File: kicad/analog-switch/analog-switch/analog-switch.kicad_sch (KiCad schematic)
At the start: 12 parts, among them J1 Conn_01x04, J2 Conn_01x16_MountingPin, J3 Conn_02x01_Row_Letter_First, J4 Conn_01x04, J5 Conn_01x16_MountingPin, Q1 Q_PNP_EBC, U1 CD74HC4067M, U2 74HC595, U3 CD74HC4067M

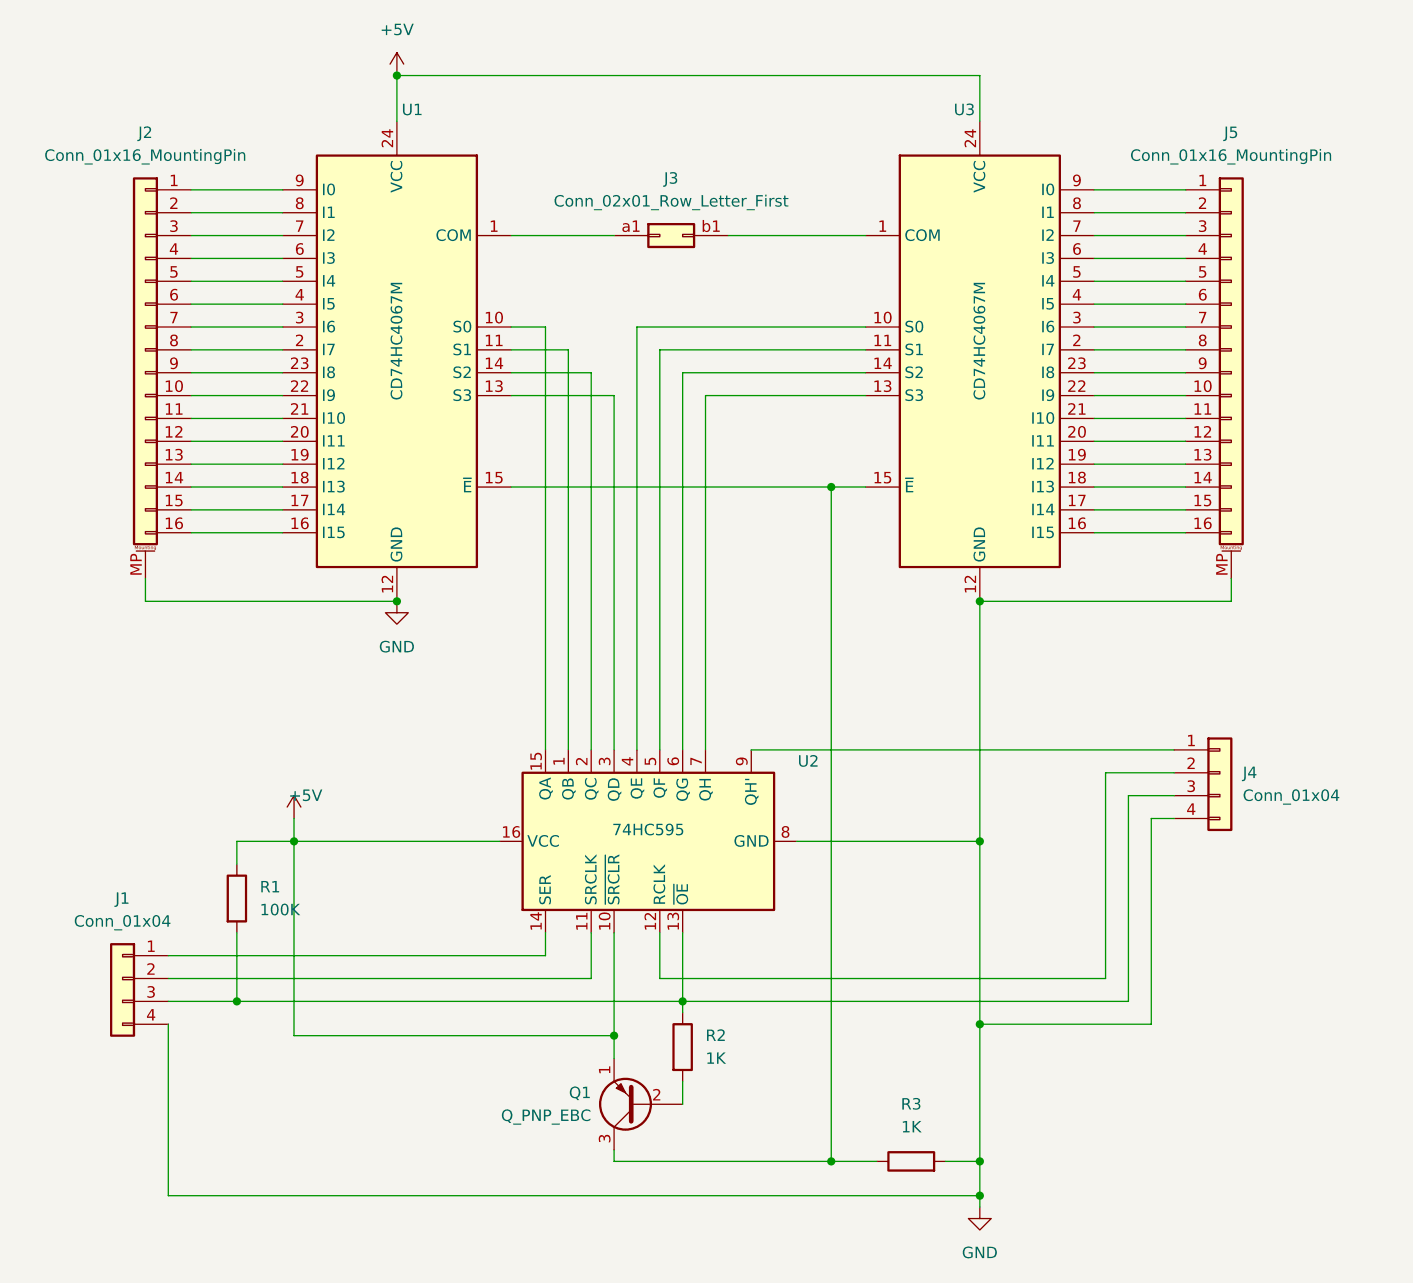
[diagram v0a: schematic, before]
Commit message: proj settings
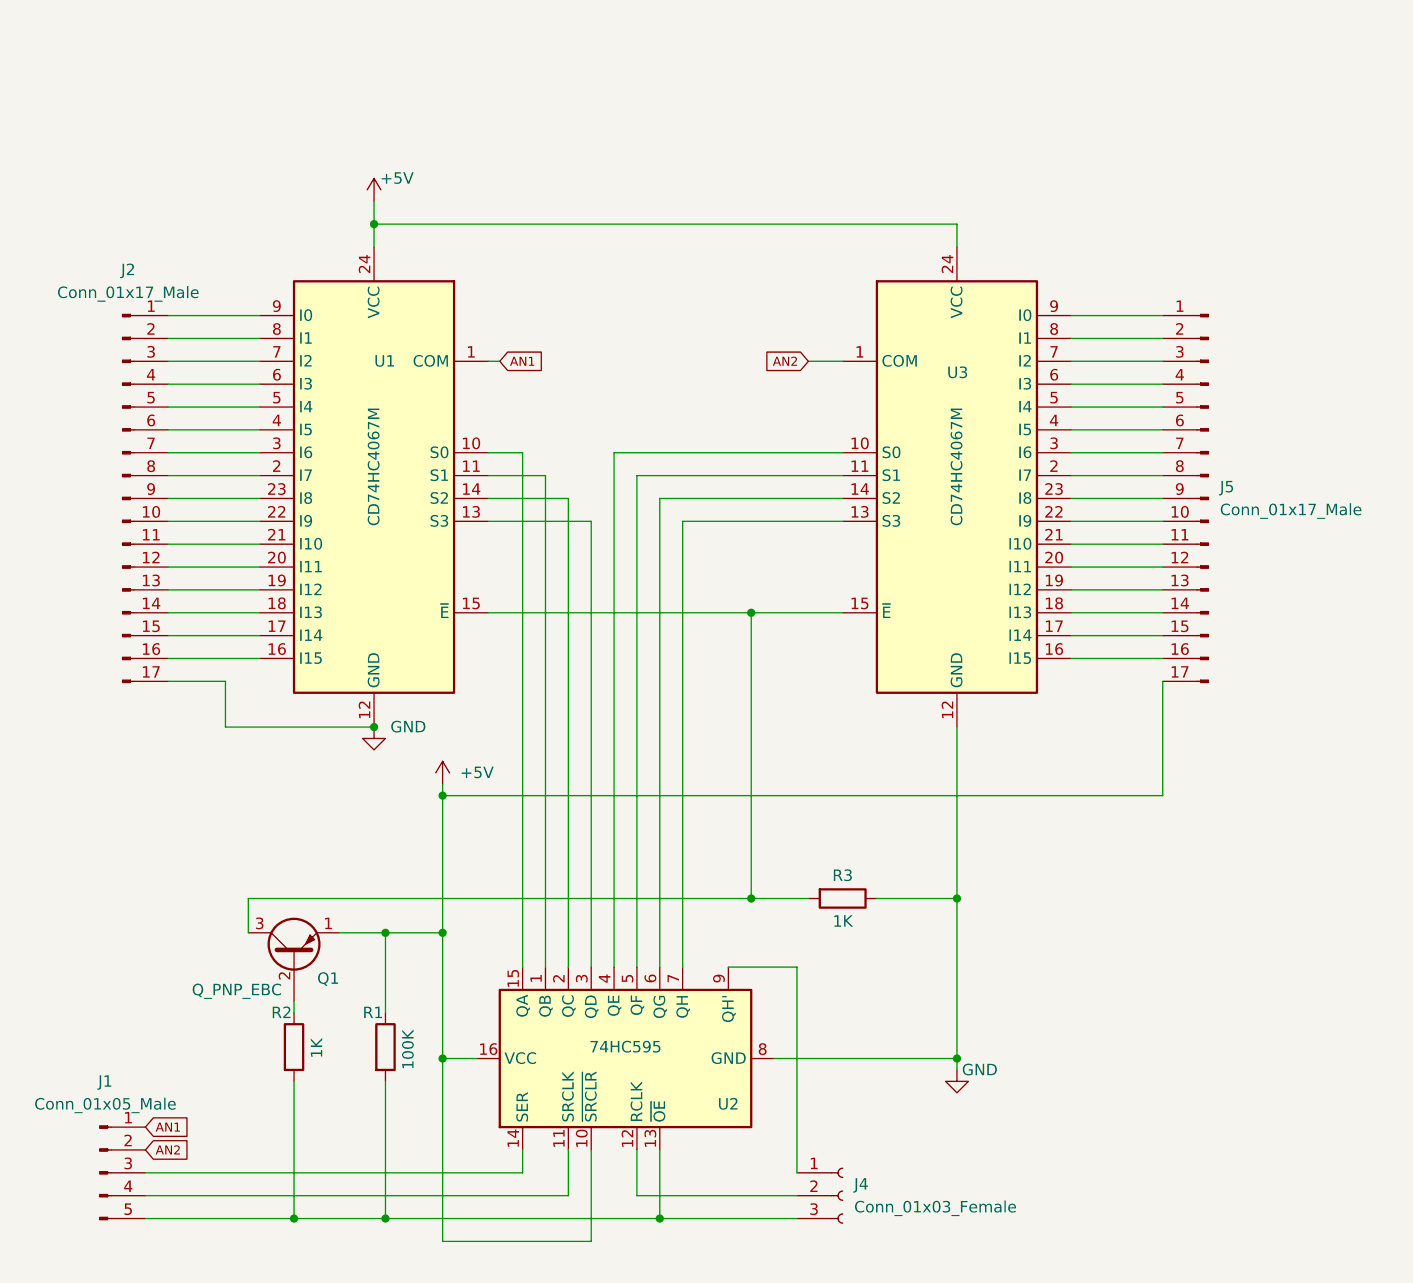
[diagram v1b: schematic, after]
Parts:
- removed J1, J4: Conn_01x04, Connector_PinHeader_2.54mm:PinHeader_1x04_P2.54mm_Vertical, symbol Connector_Generic:Conn_01x04
- removed J2, J5: Conn_01x16_MountingPin, Connector_PinHeader_2.54mm:PinHeader_1x16_P2.54mm_Vertical, symbol Connector_Generic_MountingPin:Conn_01x16_MountingPin
- removed J3: Conn_02x01_Row_Letter_First, symbol Connector_Generic:Conn_02x01_Row_Letter_First
- added J1: Conn_01x05_Male, Connector_PinHeader_2.00mm:PinHeader_1x05_P2.00mm_Vertical, symbol Connector:Conn_01x05_Male
- added J2, J5: Conn_01x17_Male, Connector_PinHeader_2.54mm:PinHeader_1x17_P2.54mm_Vertical, symbol Connector:Conn_01x17_Male
- added J4: Conn_01x03_Female, Connector_PinHeader_2.00mm:PinHeader_1x03_P2.00mm_Vertical, symbol Connector:Conn_01x03_Female
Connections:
- net +5V: now also J5.17 (Pin_17)
- net GND: now also R3.1, J2.17 (Pin_17); no longer R3.2
- net at U2.9 (QH'): now also J4.1 (Pin_1)
- net at U2.12 (RCLK): now also J4.2 (Pin_2)
- net at R1.2, U2.13 (~{OE}): now also R2.2, J1.5 (Pin_5), J4.3 (Pin_3); no longer R2.1
- net AN2: now reaches U3.1 (COM)
- net AN2: now also J1.2 (Pin_2)
- net at Q1.3 (C), U1.15 (~{E}), U3.15 (~{E}): now also R3.2; no longer R3.1
- net at U3.16 (I15): now also J5.16 (Pin_16)
- net at U3.17 (I14): now also J5.15 (Pin_15)
- net at U3.18 (I13): now also J5.14 (Pin_14)
- net at U3.19 (I12): now also J5.13 (Pin_13)
- net at U3.2 (I7): now also J5.8 (Pin_8)
- net at U3.20 (I11): now also J5.12 (Pin_12)
- net at U3.21 (I10): now also J5.11 (Pin_11)
- net at U3.22 (I9): now also J5.10 (Pin_10)
- net at U3.23 (I8): now also J5.9 (Pin_9)
- net at U3.3 (I6): now also J5.7 (Pin_7)
- net at U3.4 (I5): now also J5.6 (Pin_6)
- net at U3.5 (I4): now also J5.5 (Pin_5)
- net at U3.6 (I3): now also J5.4 (Pin_4)
- net at U3.7 (I2): now also J5.3 (Pin_3)
- net at U3.8 (I1): now also J5.2 (Pin_2)
- net at U3.9 (I0): now also J5.1 (Pin_1)
- net AN1: now reaches U1.1 (COM)
- net AN1: now also J1.1 (Pin_1)
- net at U1.16 (I15): now also J2.16 (Pin_16)
- net at U1.17 (I14): now also J2.15 (Pin_15)
- net at U1.18 (I13): now also J2.14 (Pin_14)
- net at U1.19 (I12): now also J2.13 (Pin_13)
- net at U1.2 (I7): now also J2.8 (Pin_8)
- net at U1.20 (I11): now also J2.12 (Pin_12)
- net at U1.21 (I10): now also J2.11 (Pin_11)
- net at U1.22 (I9): now also J2.10 (Pin_10)
- net at U1.23 (I8): now also J2.9 (Pin_9)
- net at U1.3 (I6): now also J2.7 (Pin_7)
- net at U1.4 (I5): now also J2.6 (Pin_6)
- net at U1.5 (I4): now also J2.5 (Pin_5)
- net at U1.6 (I3): now also J2.4 (Pin_4)
- net at U1.7 (I2): now also J2.3 (Pin_3)
- net at U1.8 (I1): now also J2.2 (Pin_2)
- net at U1.9 (I0): now also J2.1 (Pin_1)
- net at U2.11 (SRCLK): now also J1.4 (Pin_4)
- net at U2.14 (SER): now also J1.3 (Pin_3)
- net at Q1.2 (B): now also R2.1; no longer R2.2
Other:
- moved on the sheet: Q1, R1, R2, R3, U1, U2, U3
